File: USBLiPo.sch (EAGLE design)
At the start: 15 parts, among them IC1 LTC4054, J1 USB, Q1 2N7002

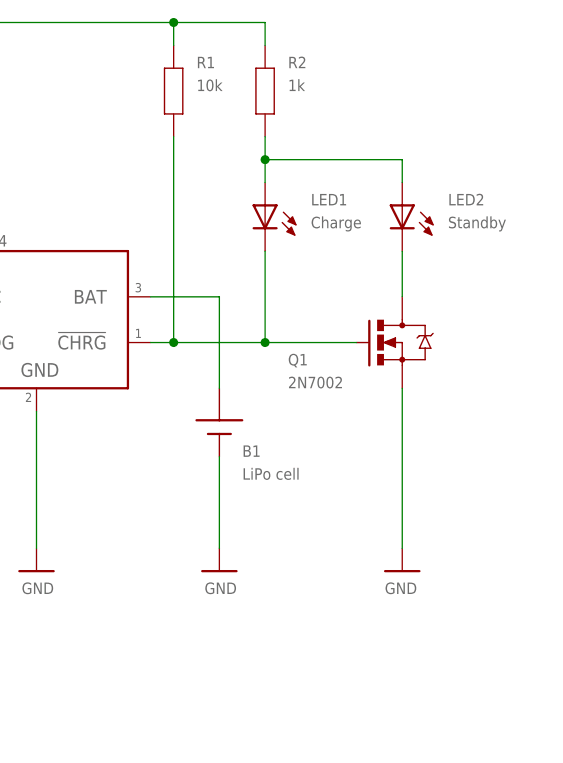
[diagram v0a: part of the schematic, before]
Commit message: foo
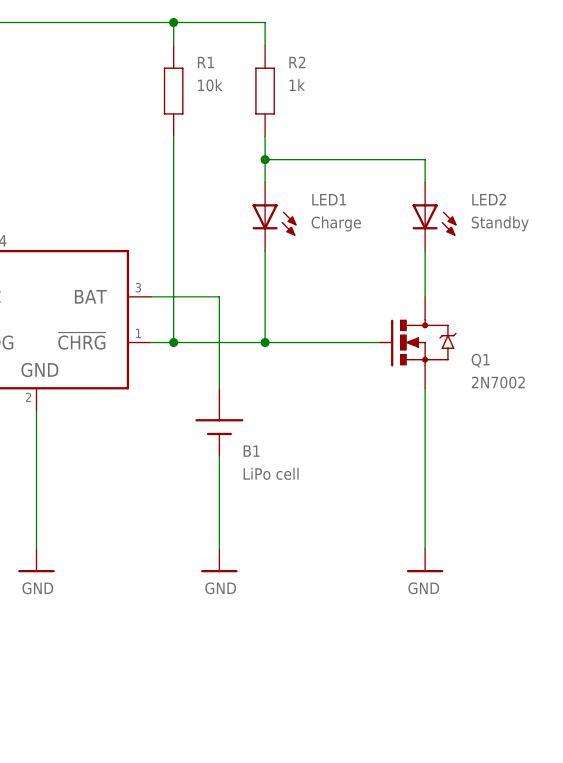
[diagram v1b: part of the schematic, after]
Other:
- note added: "2.0mm JST"
- note removed: "2-pin 2.0mm JST"
- moved on the sheet: LED2, Q1
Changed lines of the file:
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@@
 <setting verticaltext="up"/>
 </settings>
-<grid distance="0.1" unitdist="inch" unit="inch" style="lines" multiple="1" display="yes" altdistance="0.01" altunitdist="inch" altunit="inch"/>
+<grid distance="0.1" unitdist="inch" unit="inch" style="lines" multiple="1" display="no" altdistance="0.01" altunitdist="inch" altunit="inch"/>
 <layers>
 <layer number="1" name="Top" color="4" fill="1" visible="no" active="no"/>
@@
 <text x="53.34" y="86.36" size="1.27" layer="98">1812</text>
 <text x="55.88" y="55.88" size="1.27" layer="98">0603</text>
-<text x="129.54" y="58.42" size="1.27" layer="98">2-pin 2.0mm JST</text>
-<text x="134.62" y="68.58" size="1.27" layer="98">SOT-23</text>
+<text x="129.54" y="58.42" size="1.27" layer="98">2.0mm JST</text>
+<text x="154.94" y="68.58" size="1.27" layer="98">SOT-23</text>
 <text x="124.46" y="101.6" size="1.27" layer="98">0603</text>
 <text x="137.16" y="86.36" size="1.27" layer="98">0603</text>
-<text x="152.4" y="86.36" size="1.27" layer="98">0603</text>
+<text x="154.94" y="86.36" size="1.27" layer="98">0603</text>
 <text x="134.62" y="101.6" size="1.27" layer="98">0603</text>
 <text x="93.98" y="55.88" size="1.27" layer="98">0603</text>
@@
 <wire x1="134.62" y1="10.16" x2="134.62" y2="38.1" width="0.1524" layer="98"/>
 <text x="137.16" y="83.82" size="1.27" layer="98">Green</text>
-<text x="152.4" y="83.82" size="1.27" layer="98">Yellow</text>
+<text x="154.94" y="83.82" size="1.27" layer="98">Yellow</text>
+<wire x1="121.92" y1="73.66" x2="142.24" y2="73.66" width="0.3048" layer="98" style="shortdash"/>
+<wire x1="142.24" y1="73.66" x2="142.24" y2="55.88" width="0.3048" layer="98" style="shortdash"/>
+<wire x1="142.24" y1="55.88" x2="121.92" y2="55.88" width="0.3048" layer="98" style="shortdash"/>
+<wire x1="121.92" y1="55.88" x2="121.92" y2="73.66" width="0.3048" layer="98" style="shortdash"/>
 </plain>
 <instances>
@@
 </instance>
 <instance part="U$4" gate="G$1" x="63.5" y="50.8"/>
-<instance part="U$6" gate="G$1" x="147.32" y="50.8" rot="MR0"/>
+<instance part="U$6" gate="G$1" x="149.86" y="50.8" rot="MR0"/>
 <instance part="U$7" gate="G$1" x="127" y="50.8"/>
 <instance part="F1" gate="G$1" x="53.34" y="81.28" smashed="yes">
@@
 <attribute name="VALUE" x="137.16" y="88.9" size="1.27" layer="96"/>
 </instance>
-<instance part="LED2" gate="G$1" x="147.32" y="91.44" smashed="yes" rot="MR0">
-<attribute name="NAME" x="152.4" y="91.44" size="1.27" layer="95"/>
-<attribute name="VALUE" x="152.4" y="88.9" size="1.27" layer="96"/>
+<instance part="LED2" gate="G$1" x="149.86" y="91.44" smashed="yes" rot="MR0">
+<attribute name="NAME" x="154.94" y="91.44" size="1.27" layer="95"/>
+<attribute name="VALUE" x="154.94" y="88.9" size="1.27" layer="96"/>
 </instance>
 <instance part="J1" gate="G$1" x="35.56" y="76.2"/>
-<instance part="Q1" gate="G$1" x="147.32" y="76.2" smashed="yes">
-<attribute name="NAME" x="134.62" y="73.66" size="1.27" layer="95"/>
-<attribute name="VALUE" x="134.62" y="71.12" size="1.27" layer="96"/>
+<instance part="Q1" gate="G$1" x="149.86" y="76.2" smashed="yes">
+<attribute name="NAME" x="154.94" y="73.66" size="1.27" layer="95"/>
+<attribute name="VALUE" x="154.94" y="71.12" size="1.27" layer="96"/>
 </instance>
 <instance part="R3" gate="G$1" x="71.12" y="60.96" smashed="yes" rot="MR270">
@@
 </segment>
 <segment>
-<wire x1="147.32" y1="71.12" x2="147.32" y2="53.34" width="0.1524" layer="91"/>
+<wire x1="149.86" y1="71.12" x2="149.86" y2="53.34" width="0.1524" layer="91"/>
 <pinref part="U$6" gate="G$1" pin="GND"/>
 <pinref part="Q1" gate="G$1" pin="S"/>
@@
 <net name="N$1" class="0">
 <segment>
-<wire x1="147.32" y1="86.36" x2="147.32" y2="81.28" width="0.1524" layer="91"/>
+<wire x1="149.86" y1="86.36" x2="149.86" y2="81.28" width="0.1524" layer="91"/>
 <pinref part="LED2" gate="G$1" pin="C"/>
 <pinref part="Q1" gate="G$1" pin="D"/>
@@
 <net name="N$8" class="0">
 <segment>
-<wire x1="132.08" y1="96.52" x2="147.32" y2="96.52" width="0.1524" layer="91"/>
-<wire x1="147.32" y1="96.52" x2="147.32" y2="93.98" width="0.1524" layer="91"/>
+<wire x1="132.08" y1="96.52" x2="149.86" y2="96.52" width="0.1524" layer="91"/>
+<wire x1="149.86" y1="96.52" x2="149.86" y2="93.98" width="0.1524" layer="91"/>
 <wire x1="132.08" y1="93.98" x2="132.08" y2="96.52" width="0.1524" layer="91"/>
 <pinref part="LED1" gate="G$1" pin="A"/>
@@
 <net name="N$6" class="0">
 <segment>
-<wire x1="142.24" y1="76.2" x2="132.08" y2="76.2" width="0.1524" layer="91"/>
+<wire x1="144.78" y1="76.2" x2="132.08" y2="76.2" width="0.1524" layer="91"/>
 <wire x1="132.08" y1="76.2" x2="121.92" y2="76.2" width="0.1524" layer="91"/>
 <wire x1="121.92" y1="99.06" x2="121.92" y2="76.2" width="0.1524" layer="91"/>

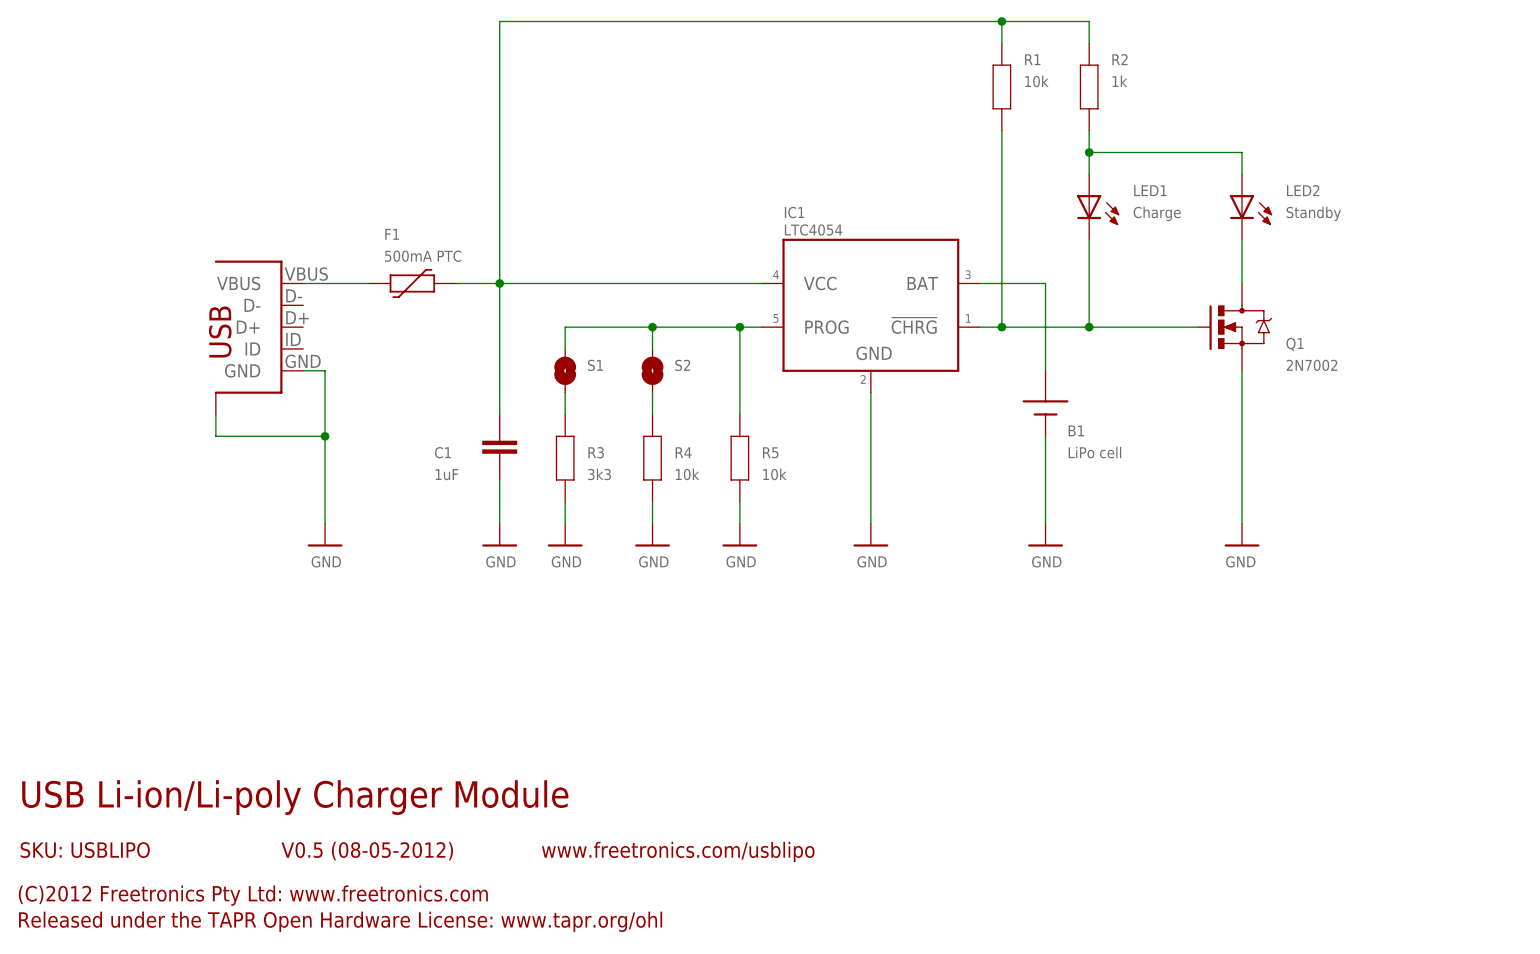
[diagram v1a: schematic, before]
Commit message: Layout and overlay
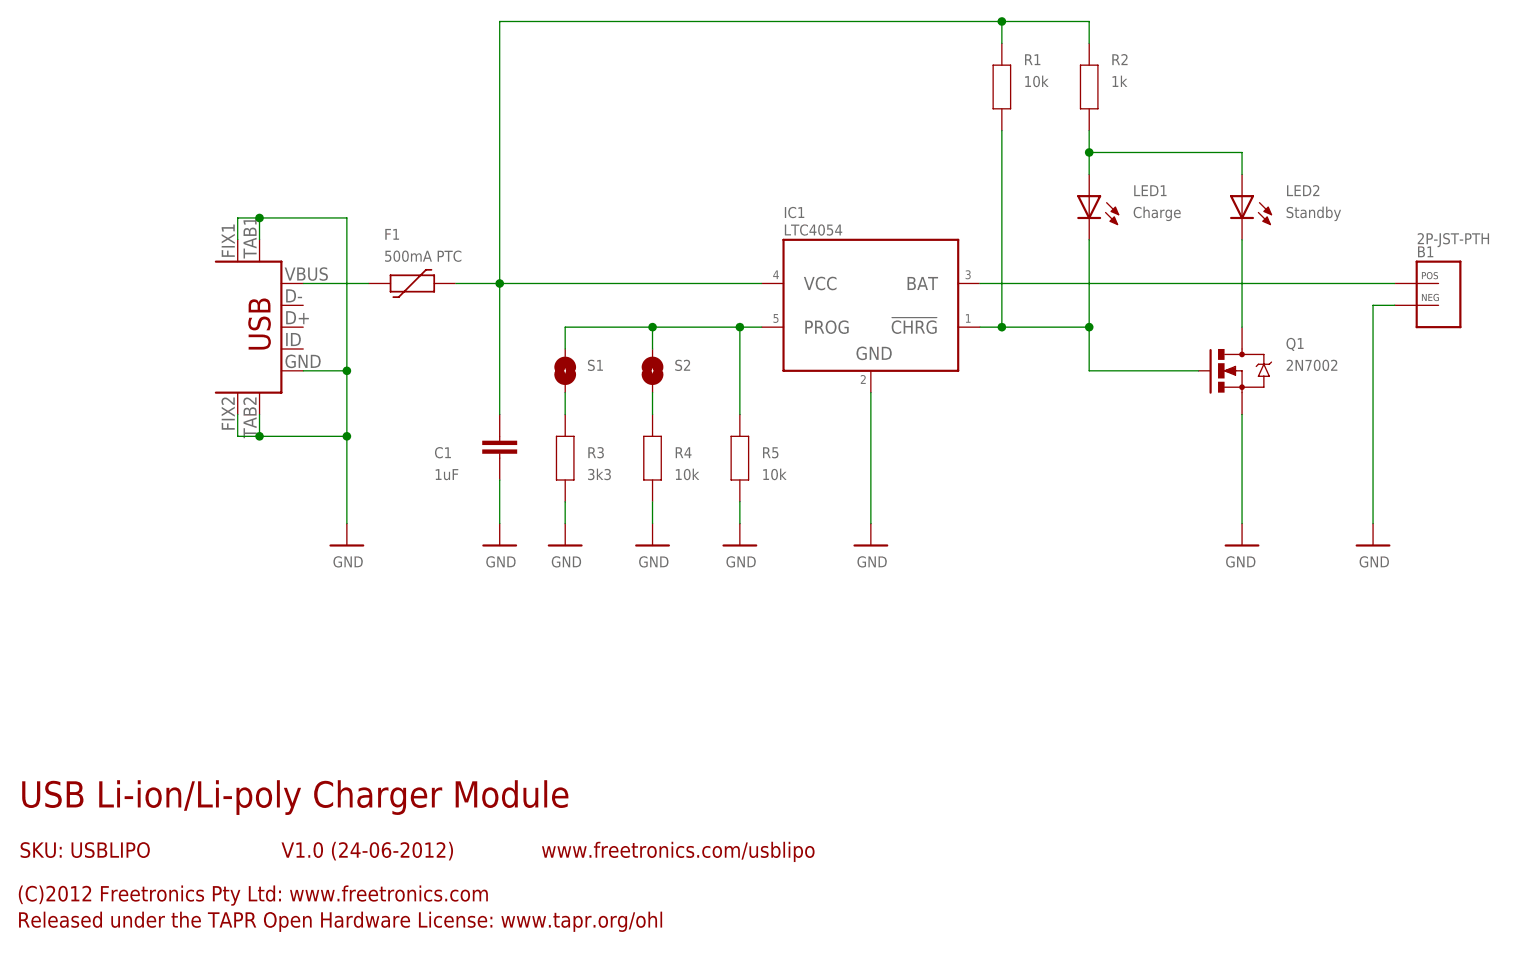
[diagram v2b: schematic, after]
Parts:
- removed J1: USB, freetronics-luke:USB-FT
- added X1: USBSF-MICROB, freetronics-jon:USBSF-MICROB
- B1: value LiPo cell -> 2P-JST-PTH; device freetronics-luke:2P-JST-TH-RA -> freetronics-jon:FREETRONICS-LUKE_2P-JST-TH-RAPTH
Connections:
- net GND: now also B1.NEG, X1.FIX1, X1.FIX2, X1.GND, X1.TAB1, X1.TAB2; no longer B1.-, J1.GND, J1.SH$1
- net N$113: now also X1.VBUS; no longer J1.VBUS
- net N$4: now also B1.POS; no longer B1.+
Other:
- note added: "SMD micro-B USB socket"
- note added: "V1.0 (24-06-2012)"
- note removed: "SMD mini-B USB socket"
- note removed: "V0.5 (08-05-2012)"
- moved on the sheet: Q1
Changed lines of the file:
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@@
 <part name="U$4" library="freetronics-luke" deviceset="GND" device=""/>
 <part name="U$6" library="freetronics-luke" deviceset="GND" device=""/>
-<part name="U$7" library="freetronics-luke" deviceset="GND" device=""/>
 <part name="F1" library="freetronics-luke" deviceset="PTC" device="" value="500mA PTC"/>
 <part name="U$2" library="freetronics-luke" deviceset="GND" device=""/>
@@
 <part name="LED1" library="freetronics-master-v1" deviceset="LED" device="0603" value="Charge"/>
 <part name="LED2" library="freetronics-master-v1" deviceset="LED" device="0603" value="Standby"/>
-<part name="J1" library="freetronics-luke" deviceset="USB-FT" device="" value="USB"/>
 <part name="Q1" library="freetronics-luke" deviceset="2N7002" device=""/>
 <part name="R3" library="freetronics" deviceset="RESISTOR" device="0603" value="3k3"/>
@@
 <part name="S1" library="freetronics-luke" deviceset="SJ" device=""/>
 <part name="S2" library="freetronics-luke" deviceset="SJ" device=""/>
-<part name="B1" library="freetronics-luke" deviceset="2P-JST-TH-RA" device="" value="LiPo cell"/>
+<part name="B1" library="freetronics-jon" deviceset="FREETRONICS-LUKE_2P-JST-TH-RA" device="PTH" value="2P-JST-PTH"/>
+<part name="U$9" library="freetronics-luke" deviceset="GND" device=""/>
+<part name="X1" library="freetronics-jon" deviceset="USBSF" device="-MICROB"/>
 </parts>
 <sheets>
@@
 <plain>
 <text x="7.62" y="20.32" size="3.048" layer="94">USB Li-ion/Li-poly Charger Module</text>
-<text x="38.1" y="14.478" size="1.778" layer="94">V0.5 (08-05-2012)</text>
+<text x="38.1" y="14.478" size="1.778" layer="94">V1.0 (24-06-2012)</text>
 <text x="7.62" y="14.478" size="1.778" layer="94">SKU: USBLIPO</text>
 <text x="7.366" y="9.398" size="1.778" layer="94">(C)2012 Freetronics Pty Ltd: www.freetronics.com</text>
 <text x="7.366" y="6.35" size="1.778" layer="94">Released under the TAPR Open Hardware License: www.tapr.org/ohl</text>
 <text x="68.326" y="14.478" size="1.778" layer="94">www.freetronics.com/usblipo</text>
-<text x="22.86" y="86.36" size="1.27" layer="98">SMD mini-B USB socket</text>
+<text x="22.86" y="91.44" size="1.27" layer="98">SMD micro-B USB socket</text>
 <text x="53.34" y="86.36" size="1.27" layer="98">1812</text>
 <text x="55.88" y="55.88" size="1.27" layer="98">0603</text>
-<text x="129.54" y="58.42" size="1.27" layer="98">2.0mm JST</text>
+<text x="170.18" y="73.66" size="1.27" layer="98">2.0mm JST</text>
 <text x="154.94" y="68.58" size="1.27" layer="98">SOT-23</text>
 <text x="124.46" y="101.6" size="1.27" layer="98">0603</text>
@@
 <text x="137.16" y="83.82" size="1.27" layer="98">Green</text>
 <text x="154.94" y="83.82" size="1.27" layer="98">Yellow</text>
-<wire x1="121.92" y1="73.66" x2="142.24" y2="73.66" width="0.3048" layer="98" style="shortdash"/>
-<wire x1="142.24" y1="73.66" x2="142.24" y2="55.88" width="0.3048" layer="98" style="shortdash"/>
-<wire x1="142.24" y1="55.88" x2="121.92" y2="55.88" width="0.3048" layer="98" style="shortdash"/>
-<wire x1="121.92" y1="55.88" x2="121.92" y2="73.66" width="0.3048" layer="98" style="shortdash"/>
 </plain>
 <instances>
@@
 <instance part="U$4" gate="G$1" x="63.5" y="50.8"/>
 <instance part="U$6" gate="G$1" x="149.86" y="50.8" rot="MR0"/>
-<instance part="U$7" gate="G$1" x="127" y="50.8"/>
 <instance part="F1" gate="G$1" x="53.34" y="81.28" smashed="yes">
 <attribute name="NAME" x="50.038" y="86.36" size="1.27" layer="95"/>
 <attribute name="VALUE" x="50.038" y="83.82" size="1.27" layer="96"/>
 </instance>
-<instance part="U$2" gate="G$1" x="43.18" y="50.8"/>
+<instance part="U$2" gate="G$1" x="45.72" y="50.8"/>
 <instance part="R5" gate="G$1" x="91.44" y="60.96" smashed="yes" rot="MR270">
 <attribute name="NAME" x="93.98" y="60.96" size="1.27" layer="95"/>
@@
 <attribute name="VALUE" x="154.94" y="88.9" size="1.27" layer="96"/>
 </instance>
-<instance part="J1" gate="G$1" x="35.56" y="76.2"/>
-<instance part="Q1" gate="G$1" x="149.86" y="76.2" smashed="yes">
+<instance part="Q1" gate="G$1" x="149.86" y="71.12" smashed="yes">
 <attribute name="NAME" x="154.94" y="73.66" size="1.27" layer="95"/>
 <attribute name="VALUE" x="154.94" y="71.12" size="1.27" layer="96"/>
@@
 <attribute name="NAME" x="83.82" y="71.12" size="1.27" layer="95"/>
 </instance>
-<instance part="B1" gate="G$1" x="127" y="66.04" smashed="yes">
-<attribute name="NAME" x="129.54" y="63.5" size="1.27" layer="95" font="vector"/>
-<attribute name="VALUE" x="129.54" y="60.96" size="1.27" layer="96"/>
-</instance>
+<instance part="B1" gate="G$1" x="170.18" y="78.74"/>
+<instance part="U$9" gate="G$1" x="165.1" y="50.8"/>
+<instance part="X1" gate="G$1" x="35.56" y="76.2" rot="R180"/>
 </instances>
 <busses>
@@
 </segment>
 <segment>
-<wire x1="149.86" y1="71.12" x2="149.86" y2="53.34" width="0.1524" layer="91"/>
+<wire x1="149.86" y1="66.04" x2="149.86" y2="53.34" width="0.1524" layer="91"/>
 <pinref part="U$6" gate="G$1" pin="GND"/>
 <pinref part="Q1" gate="G$1" pin="S"/>
 </segment>
 <segment>
-<wire x1="127" y1="53.34" x2="127" y2="63.5" width="0.1524" layer="91"/>
-<pinref part="U$7" gate="G$1" pin="GND"/>
-<pinref part="B1" gate="G$1" pin="-"/>
-</segment>
-<segment>
-<wire x1="40.64" y1="71.12" x2="43.18" y2="71.12" width="0.1524" layer="91"/>
-<wire x1="43.18" y1="71.12" x2="43.18" y2="63.5" width="0.1524" layer="91"/>
-<wire x1="43.18" y1="63.5" x2="43.18" y2="53.34" width="0.1524" layer="91"/>
-<wire x1="43.18" y1="63.5" x2="30.48" y2="63.5" width="0.1524" layer="91"/>
-<wire x1="30.48" y1="63.5" x2="30.48" y2="66.04" width="0.1524" layer="91"/>
-<junction x="43.18" y="63.5"/>
+<wire x1="40.64" y1="71.12" x2="45.72" y2="71.12" width="0.1524" layer="91"/>
+<wire x1="45.72" y1="71.12" x2="45.72" y2="63.5" width="0.1524" layer="91"/>
+<wire x1="45.72" y1="63.5" x2="45.72" y2="53.34" width="0.1524" layer="91"/>
+<wire x1="45.72" y1="63.5" x2="35.56" y2="63.5" width="0.1524" layer="91"/>
+<wire x1="35.56" y1="63.5" x2="35.56" y2="66.04" width="0.1524" layer="91"/>
+<junction x="45.72" y="63.5"/>
 <pinref part="U$2" gate="G$1" pin="GND"/>
-<pinref part="J1" gate="G$1" pin="GND"/>
-<pinref part="J1" gate="G$1" pin="SH$1"/>
+<pinref part="X1" gate="G$1" pin="TAB2"/>
+<pinref part="X1" gate="G$1" pin="GND"/>
+<pinref part="X1" gate="G$1" pin="TAB1"/>
+<wire x1="35.56" y1="86.36" x2="35.56" y2="88.9" width="0.1524" layer="91"/>
+<wire x1="35.56" y1="88.9" x2="45.72" y2="88.9" width="0.1524" layer="91"/>
+<wire x1="45.72" y1="88.9" x2="45.72" y2="71.12" width="0.1524" layer="91"/>
+<junction x="45.72" y="71.12"/>
+<pinref part="X1" gate="G$1" pin="FIX1"/>
+<wire x1="33.02" y1="86.36" x2="33.02" y2="88.9" width="0.1524" layer="91"/>
+<wire x1="33.02" y1="88.9" x2="35.56" y2="88.9" width="0.1524" layer="91"/>
+<pinref part="X1" gate="G$1" pin="FIX2"/>
+<wire x1="33.02" y1="66.04" x2="33.02" y2="63.5" width="0.1524" layer="91"/>
+<wire x1="33.02" y1="63.5" x2="35.56" y2="63.5" width="0.1524" layer="91"/>
+<junction x="35.56" y="63.5"/>
+<junction x="35.56" y="88.9"/>
 </segment>
 <segment>
@@
 <wire x1="81.28" y1="55.88" x2="81.28" y2="53.34" width="0.1524" layer="91"/>
 </segment>
+<segment>
+<pinref part="B1" gate="G$1" pin="NEG"/>
+<wire x1="167.64" y1="78.74" x2="165.1" y2="78.74" width="0.1524" layer="91"/>
+<wire x1="165.1" y1="78.74" x2="165.1" y2="53.34" width="0.1524" layer="91"/>
+<pinref part="U$9" gate="G$1" pin="GND"/>
+</segment>
 </net>
 <net name="N$1" class="0">
 <segment>
-<wire x1="149.86" y1="86.36" x2="149.86" y2="81.28" width="0.1524" layer="91"/>
+<wire x1="149.86" y1="86.36" x2="149.86" y2="76.2" width="0.1524" layer="91"/>
 <pinref part="LED2" gate="G$1" pin="C"/>
 <pinref part="Q1" gate="G$1" pin="D"/>
@@
 <wire x1="40.64" y1="81.28" x2="48.26" y2="81.28" width="0.1524" layer="91"/>
 <pinref part="F1" gate="G$1" pin="P$1"/>
-<pinref part="J1" gate="G$1" pin="VBUS"/>
+<pinref part="X1" gate="G$1" pin="VBUS"/>
 </segment>
 </net>
@@
 <net name="N$6" class="0">
 <segment>
-<wire x1="144.78" y1="76.2" x2="132.08" y2="76.2" width="0.1524" layer="91"/>
+<wire x1="144.78" y1="71.12" x2="132.08" y2="71.12" width="0.1524" layer="91"/>
+<wire x1="132.08" y1="71.12" x2="132.08" y2="76.2" width="0.1524" layer="91"/>
 <wire x1="132.08" y1="76.2" x2="121.92" y2="76.2" width="0.1524" layer="91"/>
 <wire x1="121.92" y1="99.06" x2="121.92" y2="76.2" width="0.1524" layer="91"/>
@@
 <net name="N$4" class="0">
 <segment>
-<wire x1="119.38" y1="81.28" x2="127" y2="81.28" width="0.1524" layer="91"/>
 <pinref part="IC1" gate="G$1" pin="BAT"/>
-<pinref part="B1" gate="G$1" pin="+"/>
-<wire x1="127" y1="81.28" x2="127" y2="71.12" width="0.1524" layer="91"/>
-</segment>
-</net>
+<pinref part="B1" gate="G$1" pin="POS"/>
+<wire x1="119.38" y1="81.28" x2="167.64" y2="81.28" width="0.1524" layer="91"/>
+</segment>
+</net>
